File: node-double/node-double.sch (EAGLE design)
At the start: 29 parts, among them IC1 TP4056, IC3 24C02, U1 ATMEGA328P_TQFP, U2 3.3V/150mA

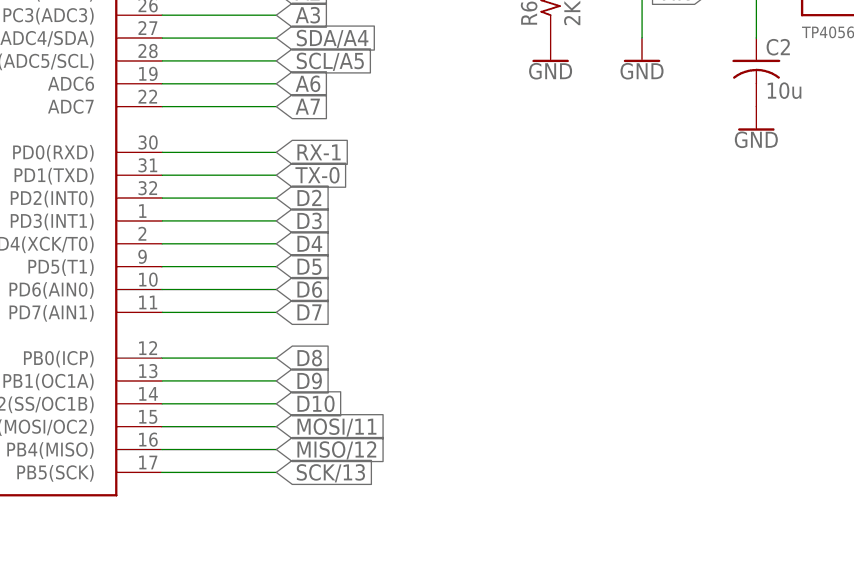
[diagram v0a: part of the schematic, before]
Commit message: Node: v4
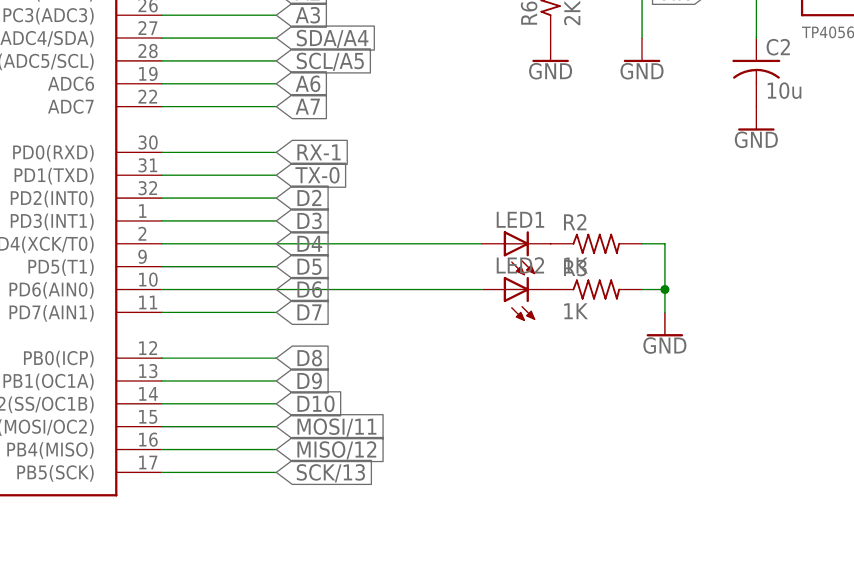
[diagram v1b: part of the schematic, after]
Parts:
- added LED1, LED2: (no value), led:LEDSML0805
- added R2, R3: 1K, resistor:R-US_R0603
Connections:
- new net N$1: LED1.C, R2.1
- new net N$2: LED2.C, R3.1
- net D4: now also LED1.A
- net D6: now also LED2.A
- net GND: now also R2.2, R3.2
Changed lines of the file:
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@@
 <part name="GND10" library="SparkFun-PowerSymbols" deviceset="GND" device=""/>
 <part name="U$2" library="pinhead" library_urn="urn:adsk.eagle:library:325" deviceset="PINHD-2X4" device="" package3d_urn="urn:adsk.eagle:package:22461/2"/>
+<part name="LED1" library="led" library_urn="urn:adsk.eagle:library:259" deviceset="LED" device="SML0805" package3d_urn="urn:adsk.eagle:package:15830/1"/>
+<part name="LED2" library="led" library_urn="urn:adsk.eagle:library:259" deviceset="LED" device="SML0805" package3d_urn="urn:adsk.eagle:package:15830/1"/>
+<part name="R2" library="resistor" library_urn="urn:adsk.eagle:library:348" deviceset="R-US_" device="R0603" package3d_urn="urn:adsk.eagle:package:26057/1" value="1K">
+<attribute name="MF" value=""/>
+<attribute name="MPN" value=""/>
+<attribute name="OC_FARNELL" value="unknown"/>
+</part>
+<part name="R3" library="resistor" library_urn="urn:adsk.eagle:library:348" deviceset="R-US_" device="R0603" package3d_urn="urn:adsk.eagle:package:26057/1" value="1K">
+<attribute name="MF" value=""/>
+<attribute name="MPN" value=""/>
+<attribute name="OC_FARNELL" value="unknown"/>
+</part>
+<part name="GND12" library="SparkFun-PowerSymbols" deviceset="GND" device=""/>
 </parts>
 <sheets>
@@
 <instance part="GND10" gate="1" x="195.58" y="-48.26"/>
 <instance part="U$2" gate="A" x="91.44" y="-7.62"/>
+<instance part="LED1" gate="G$1" x="93.98" y="53.34" rot="R90"/>
+<instance part="LED2" gate="G$1" x="93.98" y="48.26" rot="R90"/>
+<instance part="R2" gate="G$1" x="104.14" y="53.34">
+<attribute name="OC_FARNELL" x="104.14" y="53.34" size="1.778" layer="96" rot="R90" display="off"/>
+<attribute name="MF" x="104.14" y="53.34" size="1.778" layer="96" rot="R90" display="off"/>
+<attribute name="MPN" x="104.14" y="53.34" size="1.778" layer="96" rot="R90" display="off"/>
+</instance>
+<instance part="R3" gate="G$1" x="104.14" y="48.26">
+<attribute name="OC_FARNELL" x="104.14" y="48.26" size="1.778" layer="96" rot="R90" display="off"/>
+<attribute name="MF" x="104.14" y="48.26" size="1.778" layer="96" rot="R90" display="off"/>
+<attribute name="MPN" x="104.14" y="48.26" size="1.778" layer="96" rot="R90" display="off"/>
+</instance>
+<instance part="GND12" gate="1" x="111.76" y="43.18"/>
 </instances>
 <busses>
@@
 <wire x1="101.6" y1="-10.16" x2="96.52" y2="-10.16" width="0.1524" layer="91"/>
 <label x="101.6" y="-10.16" size="1.778" layer="95"/>
+</segment>
+<segment>
+<pinref part="R3" gate="G$1" pin="2"/>
+<pinref part="GND12" gate="1" pin="GND"/>
+<wire x1="109.22" y1="48.26" x2="111.76" y2="48.26" width="0.1524" layer="91"/>
+<wire x1="111.76" y1="48.26" x2="111.76" y2="45.72" width="0.1524" layer="91"/>
+<pinref part="R2" gate="G$1" pin="2"/>
+<wire x1="109.22" y1="53.34" x2="111.76" y2="53.34" width="0.1524" layer="91"/>
+<wire x1="111.76" y1="53.34" x2="111.76" y2="48.26" width="0.1524" layer="91"/>
+<junction x="111.76" y="48.26"/>
 </segment>
 </net>
@@
 <segment>
 <pinref part="U1" gate="U$1" pin="PD4(XCK/T0)"/>
-<wire x1="55.88" y1="53.34" x2="68.58" y2="53.34" width="0.1524" layer="91"/>
 <label x="68.58" y="53.34" size="1.778" layer="95" xref="yes"/>
+<pinref part="LED1" gate="G$1" pin="A"/>
+<wire x1="91.44" y1="53.34" x2="55.88" y2="53.34" width="0.1524" layer="91"/>
 </segment>
 </net>
@@
 <segment>
 <pinref part="U1" gate="U$1" pin="PD6(AIN0)"/>
-<wire x1="55.88" y1="48.26" x2="68.58" y2="48.26" width="0.1524" layer="91"/>
 <label x="68.58" y="48.26" size="1.778" layer="95" xref="yes"/>
+<pinref part="LED2" gate="G$1" pin="A"/>
+<wire x1="91.44" y1="48.26" x2="55.88" y2="48.26" width="0.1524" layer="91"/>
 </segment>
 </net>
@@
 </segment>
 </net>
+<net name="N$1" class="0">
+<segment>
+<pinref part="LED1" gate="G$1" pin="C"/>
+<pinref part="R2" gate="G$1" pin="1"/>
+</segment>
+</net>
+<net name="N$2" class="0">
+<segment>
+<pinref part="LED2" gate="G$1" pin="C"/>
+<pinref part="R3" gate="G$1" pin="1"/>
+</segment>
+</net>
